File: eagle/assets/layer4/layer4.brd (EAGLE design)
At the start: 197 x 149.4 mm, 45 parts, among them Y1 8MHz

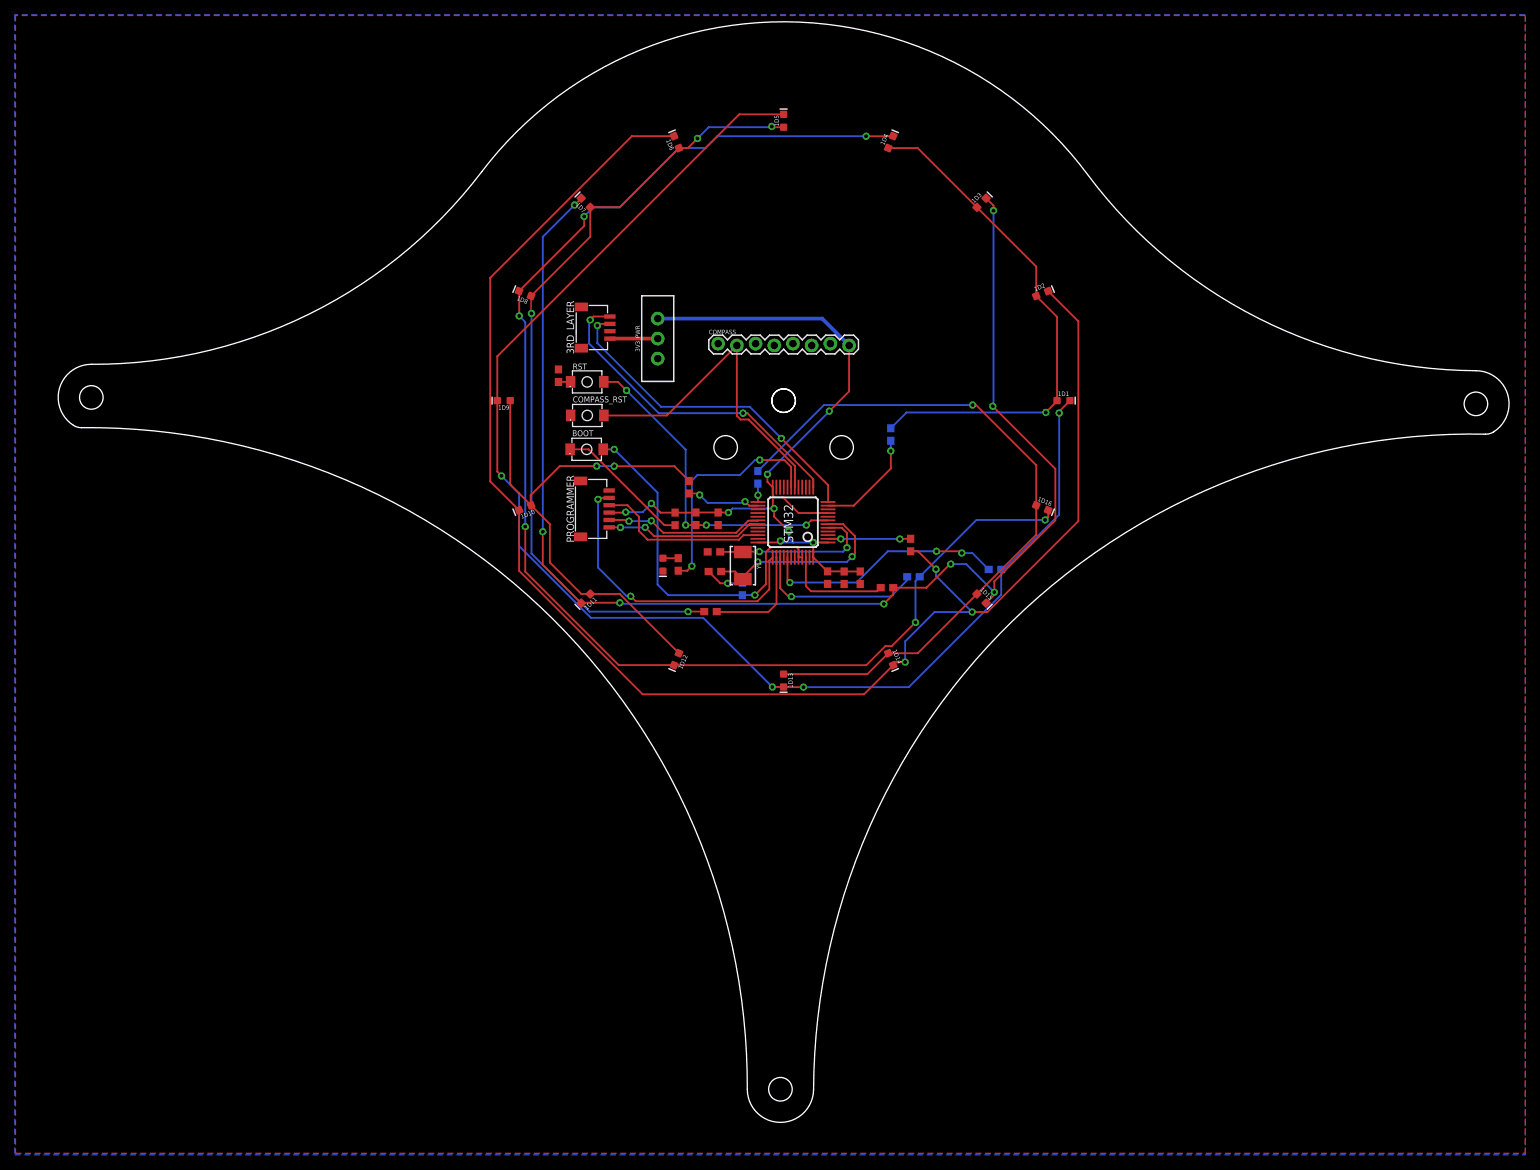
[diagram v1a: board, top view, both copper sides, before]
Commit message: 🦅 Included Layer 4 new
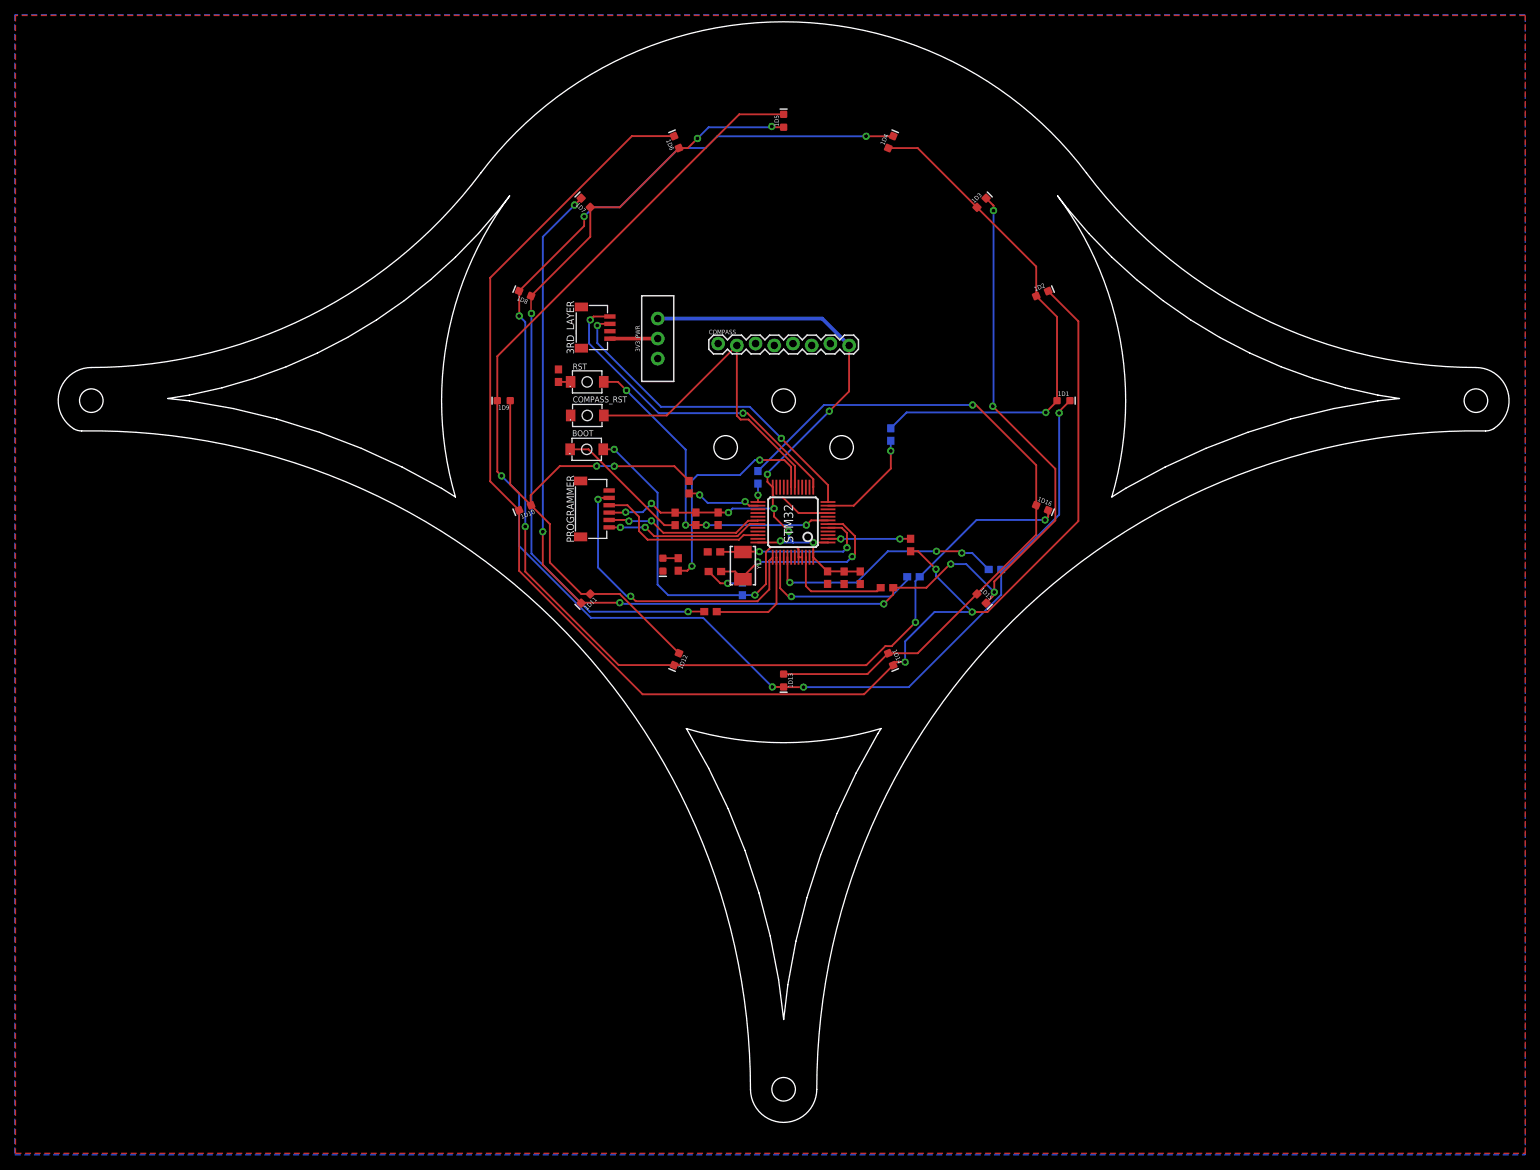
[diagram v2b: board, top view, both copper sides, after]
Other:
- outline, holes or cut-outs redrawn
